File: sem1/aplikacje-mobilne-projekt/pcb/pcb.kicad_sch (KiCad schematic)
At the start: 5 parts

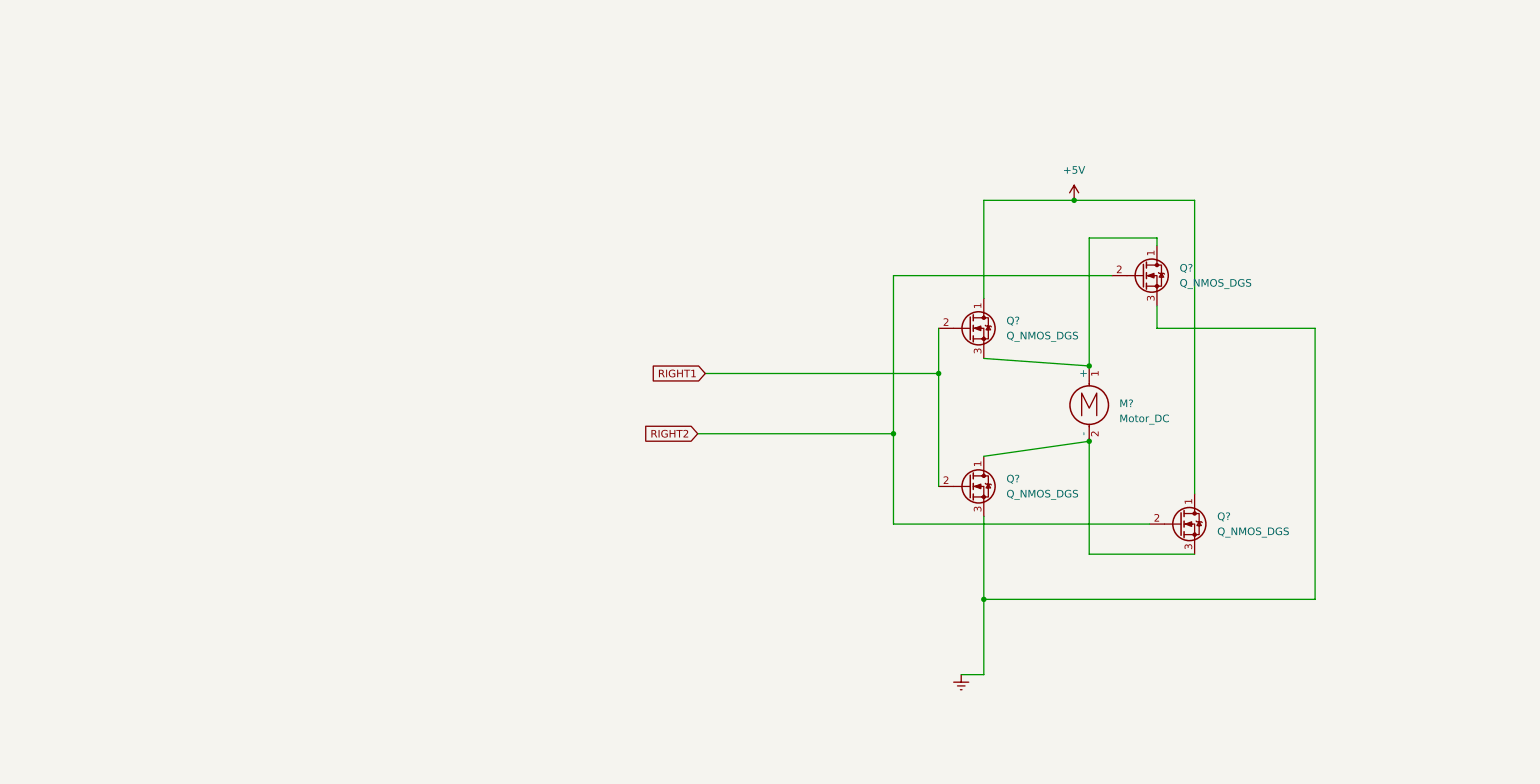
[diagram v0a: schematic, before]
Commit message: aplikacje mobilne kicad schematic
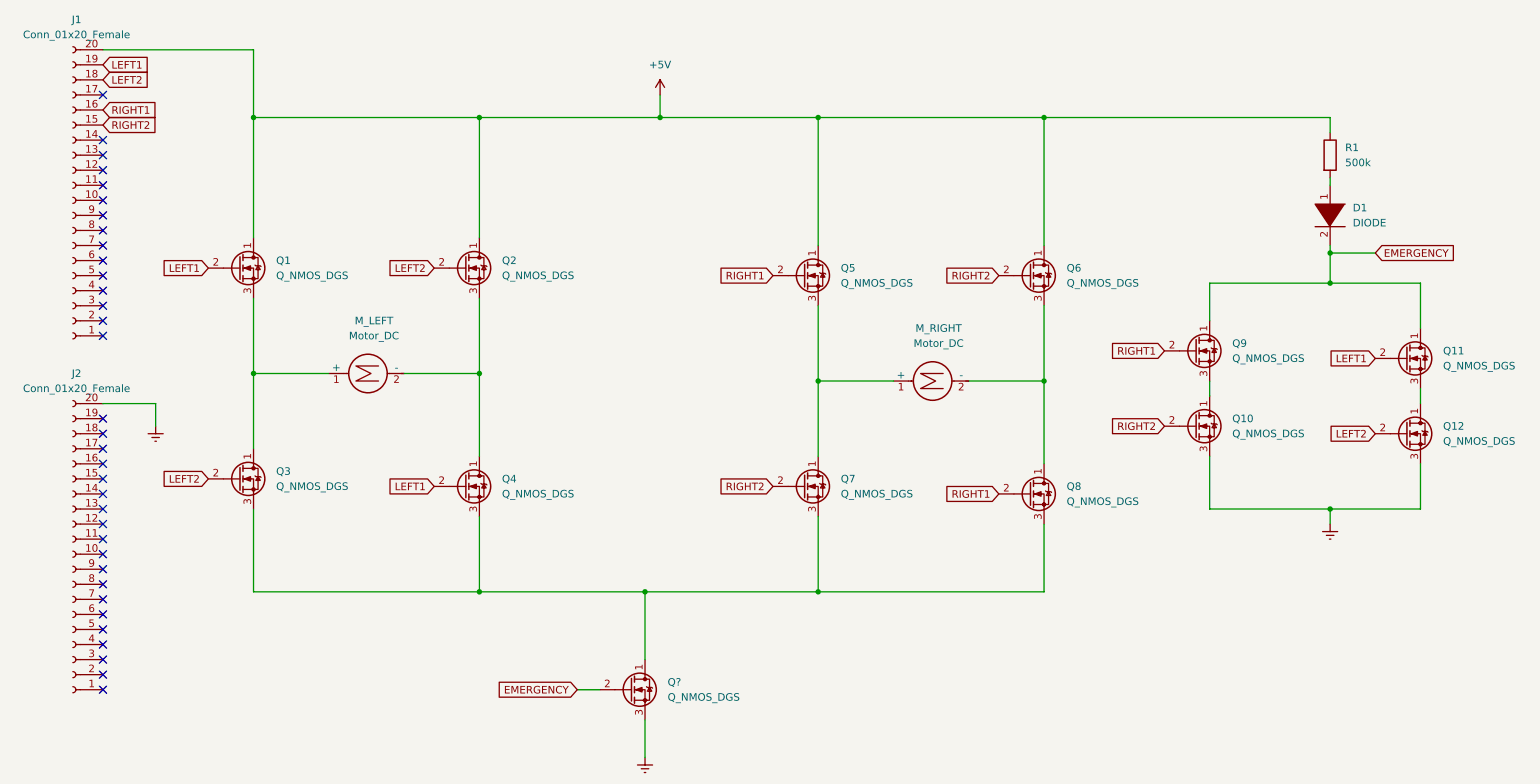
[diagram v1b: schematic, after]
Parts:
- added D1: DIODE, symbol pspice:DIODE
- added J1, J2: Conn_01x20_Female, symbol Connector:Conn_01x20_Female
- added M_LEFT: Motor_DC, symbol Motor:Motor_DC
- added Q1, Q10, Q11, Q12, Q2, Q3, Q4, Q9, Q?: Q_NMOS_DGS, symbol Device:Q_NMOS_DGS
- added R1: 500k, symbol Device:R
- gave numbers to parts that had none: 5
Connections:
- net +5V: now also Q6.1 (D), J1.20 (Pin_20), Q1.1 (D), Q2.1 (D), R1.1; no longer Q8.1 (D)
- net Earth: now also J2.20 (Pin_20), Q10.3 (S), Q12.3 (S), Q?.3 (S); no longer Q6.3 (S), Q7.3 (S)
- net RIGHT1: now also Q8.2 (G), J1.16 (Pin_16), Q9.2 (G); no longer Q7.2 (G)
- net RIGHT2: now also Q7.2 (G), J1.15 (Pin_15), Q10.2 (G); no longer Q8.2 (G)
- net at M_RIGHT.1 (+), Q5.3 (S): now also Q7.1 (D); no longer Q6.1 (D)
- new net: M_LEFT.1 (+), Q1.3 (S), Q3.1 (D)
- new net: Q3.3 (S), Q4.3 (S), Q7.3 (S), Q8.3 (S), Q?.1 (D)
- new net: M_RIGHT.2 (-), Q6.3 (S), Q8.1 (D)
- new net: D1.1 (K), R1.2
- new net: Q10.1 (D), Q9.3 (S)
- new net: Q11.3 (S), Q12.1 (D)
- new net: M_LEFT.2 (-), Q2.3 (S), Q4.1 (D)
- new net EMERGENCY: D1.2 (A), Q11.1 (D), Q9.1 (D), Q?.2 (G)
- new net LEFT1: J1.19 (Pin_19), Q1.2 (G), Q11.2 (G), Q4.2 (G)
- new net LEFT2: J1.18 (Pin_18), Q12.2 (G), Q2.2 (G), Q3.2 (G)
- no-connect marks 0 -> 34
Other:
- moved on the sheet: M_RIGHT, Q5, Q6, Q7, Q8
